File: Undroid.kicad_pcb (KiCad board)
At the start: 4 copper layers, 96 x 107.8 mm, 45 parts

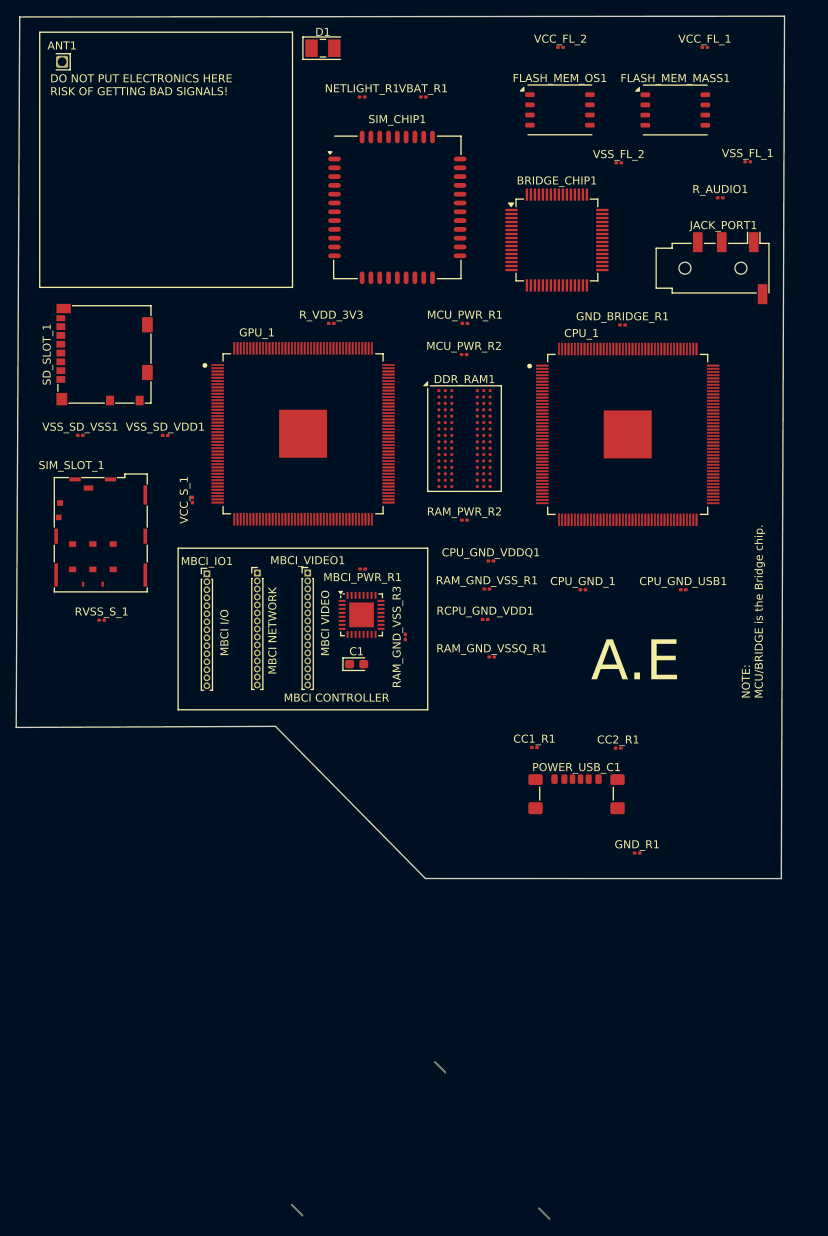
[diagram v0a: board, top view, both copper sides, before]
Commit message: board: major improvements.
Signed-off-by: Amlal EL Mahrouss <amlalelmahrouss@icloud.com>
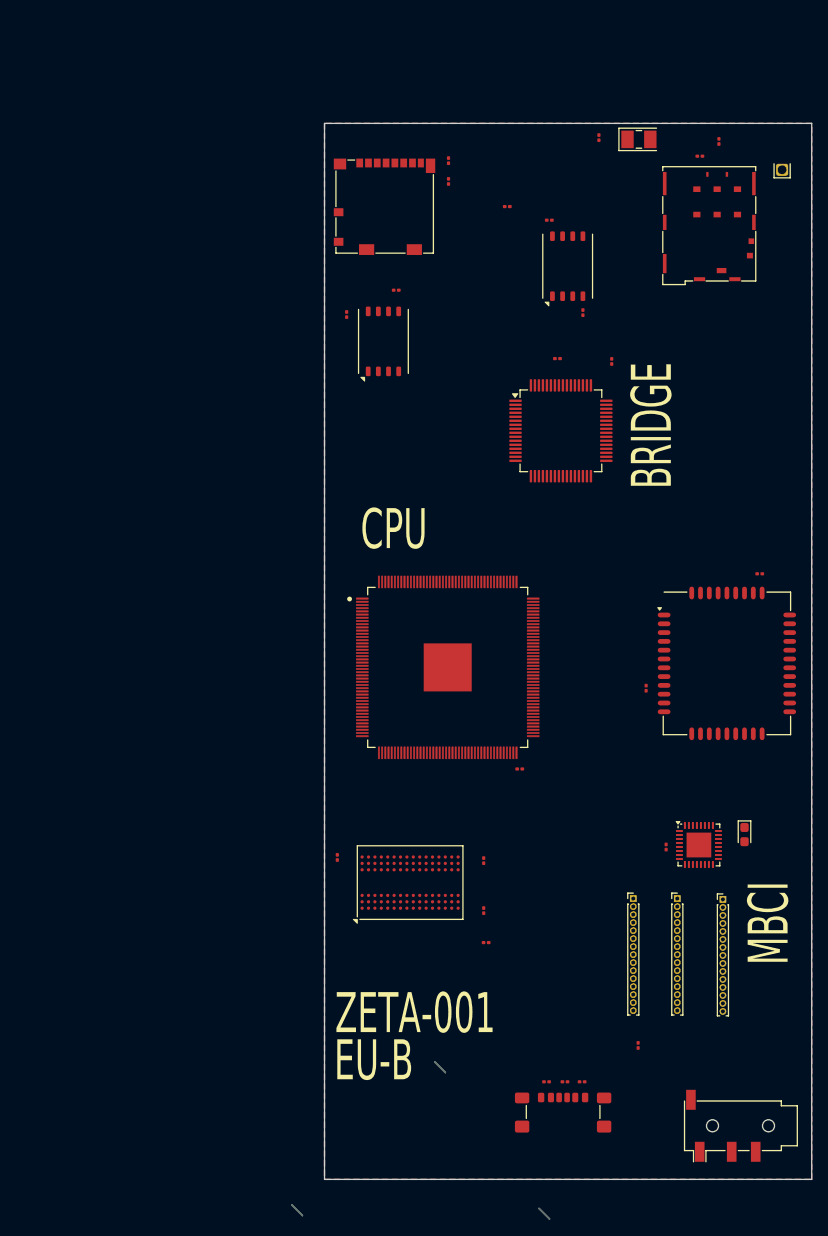
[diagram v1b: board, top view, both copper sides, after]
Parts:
- removed CPU_GND_USB1, CPU_GND_VDDQ1, RCPU_GND_VDD1: R, Resistor_SMD:R_0201_0603Metric
- removed GPU_1: Allwinner-A13, Allwinner:QFP40P2200X2200X160-177N
- moved JACK_PORT1 107.2 mm to (176.5, 155.1), turned to 180 degrees
- moved R_AUDIO1 106.5 mm to (165.0, 145.1), turned to 90 degrees
- moved RVSS_S_1 97.6 mm to (175.1, 32.1), turned to 90 degrees
- moved ANT1 91.0 mm to (183.0, 35.6), turned to 90 degrees
- moved SIM_SLOT_1 88.9 mm to (174.9, 40.5), turned to 0 degrees
- moved VCC_S_1 76.6 mm to (172.7, 33.9), turned to 0 degrees
- moved VBAT_R1 72.9 mm to (180.2, 86.1)
- moved SIM_CHIP1 70.3 mm to (176.1, 97.3)
- moved MBCI_IO1 67.0 mm to (164.4, 126.7)
- moved MBCI_NETWORK1 66.4 mm to (169.9, 126.7)
- moved MBCI_VIDEO1 66.0 mm to (175.6, 126.8)
- moved R_VDD_3V3 60.2 mm to (166.0, 100.4), turned to 90 degrees
- moved VSS_SD_VSS1 55.9 mm to (141.3, 37.1), turned to 90 degrees
- moved DDR_RAM1 55.9 mm to (136.5, 124.7), turned to 90 degrees
- moved C1 53.0 mm to (178.3, 118.7), turned to -90 degrees
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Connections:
- BRIDGE_CHIP1 pad 2: A14 -> RAM_BA2
- BRIDGE_CHIP1 pad 20: A12/BC_N -> RAM_BA0
- BRIDGE_CHIP1 pad 21: A13 -> RAM_BA1
- BRIDGE_CHIP1 pad 37: PWR_TST -> unconnected-(BRIDGE_CHIP1-TST-Pad37)
- BRIDGE_CHIP1 pad 46: TX2 -> unconnected-(BRIDGE_CHIP1-PB4-Pad46)
- BRIDGE_CHIP1 pad 47: RX2 -> unconnected-(BRIDGE_CHIP1-PB5-Pad47)
- MBCI_0 pad 11: unconnected-(MBCI_0-PD1-Pad11) -> A11
- MBCI_0 pad 12: unconnected-(MBCI_0-PD2-Pad12) -> A12/BC_N
- MBCI_0 pad 13: unconnected-(MBCI_0-PD3-Pad13) -> A13
- MBCI_0 pad 14: unconnected-(MBCI_0-PD4-Pad14) -> A14
- MBCI_0 pad 15: unconnected-(MBCI_0-PD5-Pad15) -> RAM_BA2
- MBCI_0 pad 16: unconnected-(MBCI_0-PD6-Pad16) -> RAM_BA1
- MBCI_0 pad 17: unconnected-(MBCI_0-VREFA/PD7-Pad17) -> RAM_BA0
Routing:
- added copper zone on B.Cu, net GND
- added copper zone on F.Cu, net GND
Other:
- board size 96 x 107.8 mm -> 60.9 x 132 mm
- copper layers 4 -> 2
- board text added: "BRIDGE"
- board text added: "CPU"
- board text added: "EU-B"
- board text added: "MBCI"
- board text added: "ZETA-001"
- board text removed: "A.E"
- board text removed: "DO NOT PUT ELECTRONICS HERE RISK OF GETTING BAD SIGNALS!"
- board text removed: "MBCI CONTROLLER"
- board text removed: "MBCI I/O"
- board text removed: "MBCI NETWORK"
- board text removed: "MBCI VIDEO"
- board text removed: "NOTE: MCU/BRIDGE is the Bridge chip."
